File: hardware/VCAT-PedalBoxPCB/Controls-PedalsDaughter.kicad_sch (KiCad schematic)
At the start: 26 parts, among them J1 MX150_02x03_Vertical, J3 Conn_02x03_Top_Bottom, J4 Conn_02x06_Top_Bottom, J5 Conn_02x04_Top_Bottom, J6 MX150_02x10_Vertical

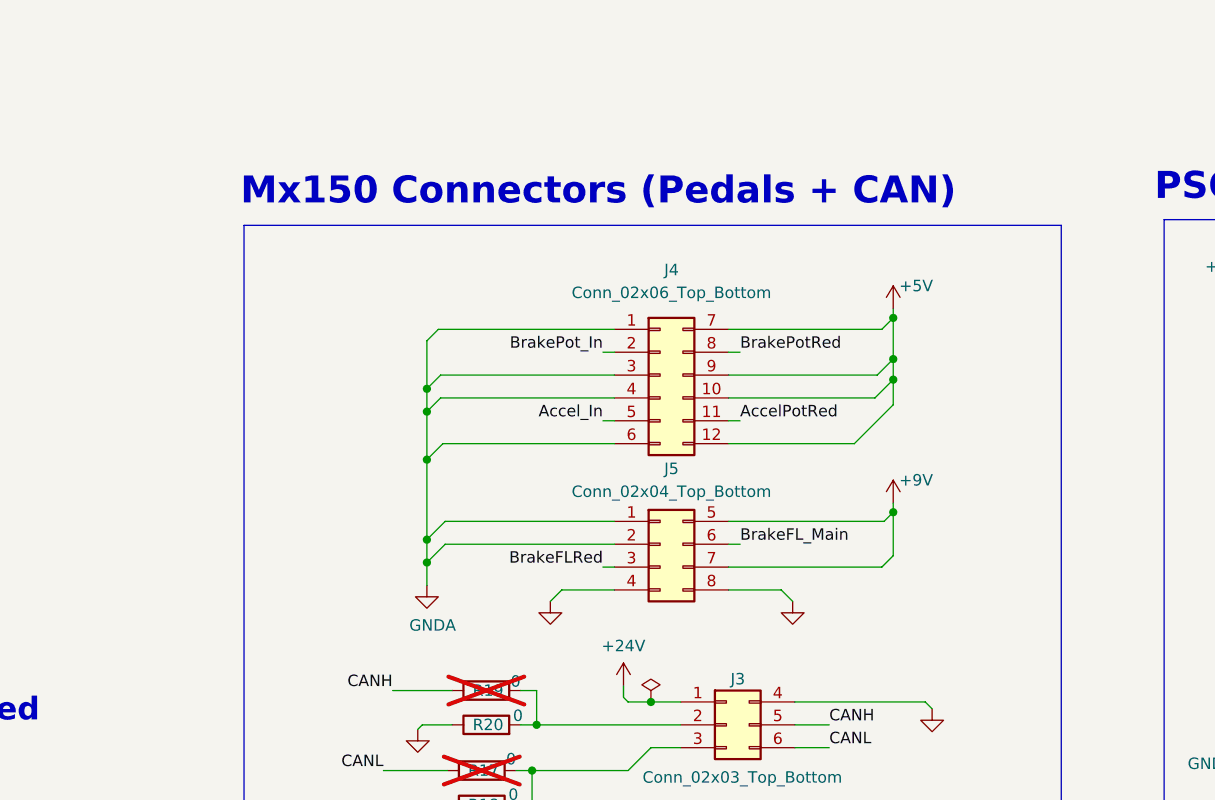
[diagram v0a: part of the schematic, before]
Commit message: Rev B - Layout Review
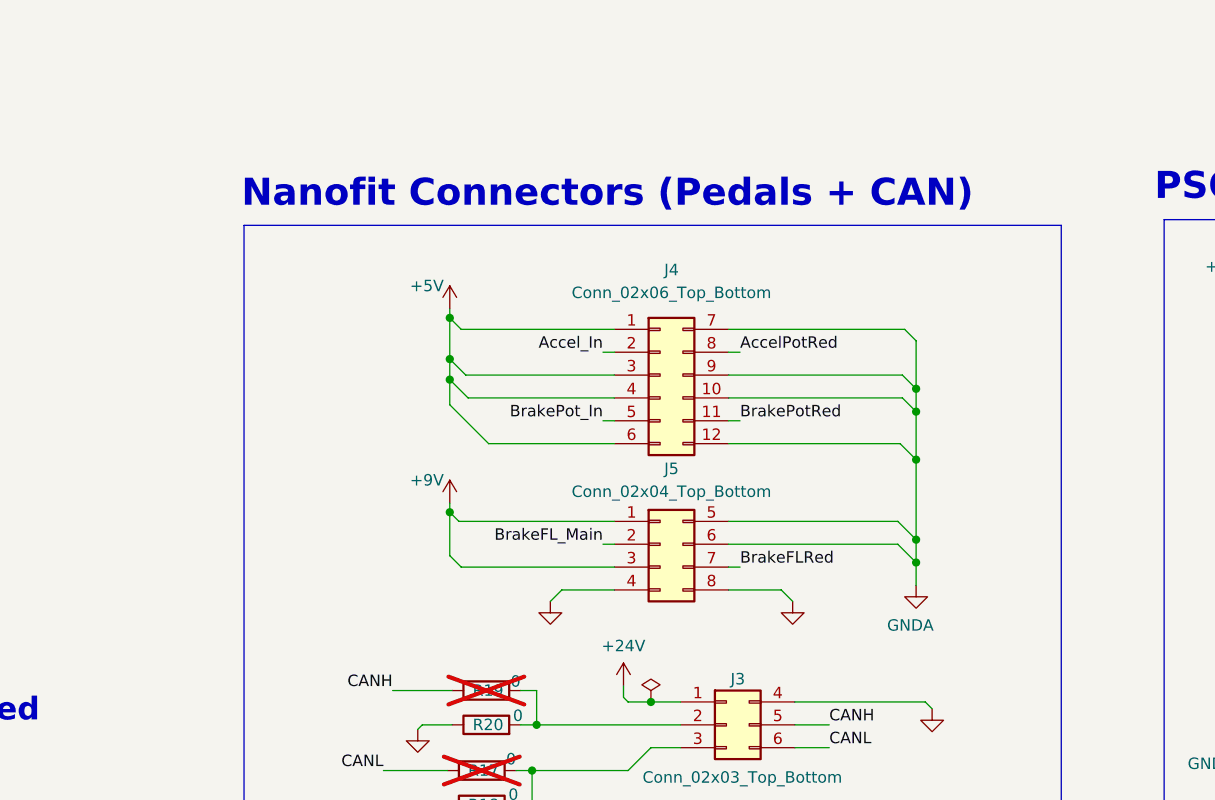
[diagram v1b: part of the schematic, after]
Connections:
- net +5V: now also J4.1 (Pin_1), J4.3 (Pin_3), J4.4 (Pin_4), J4.6 (Pin_6); no longer J4.10 (Pin_10), J4.12 (Pin_12), J4.7 (Pin_7), J4.9 (Pin_9)
- net +9V: now also J5.1 (Pin_1), J5.3 (Pin_3); no longer J5.5 (Pin_5), J5.7 (Pin_7)
- net AccelPotRed: now also J4.8 (Pin_8); no longer J4.11 (Pin_11)
- net Accel_In: now also J4.2 (Pin_2); no longer J4.5 (Pin_5)
- net BrakeFLRed: now also J5.7 (Pin_7); no longer J5.3 (Pin_3)
- net BrakeFL_Main: now also J5.2 (Pin_2); no longer J5.6 (Pin_6)
- net BrakePotRed: now also J4.11 (Pin_11); no longer J4.8 (Pin_8)
- net BrakePot_In: now also J4.5 (Pin_5); no longer J4.2 (Pin_2)
- net GNDA: now also J4.10 (Pin_10), J4.12 (Pin_12), J4.7 (Pin_7), J4.9 (Pin_9), J5.5 (Pin_5), J5.6 (Pin_6); no longer J4.1 (Pin_1), J4.3 (Pin_3), J4.4 (Pin_4), J4.6 (Pin_6), J5.1 (Pin_1), J5.2 (Pin_2)
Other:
- note added: "Nanofit Connectors (Pedals + CAN)"
- note removed: "Mx150 Connectors (Pedals + CAN)"
